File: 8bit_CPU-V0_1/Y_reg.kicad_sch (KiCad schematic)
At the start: 3 parts, among them U38 74LS04, U60 74LS574

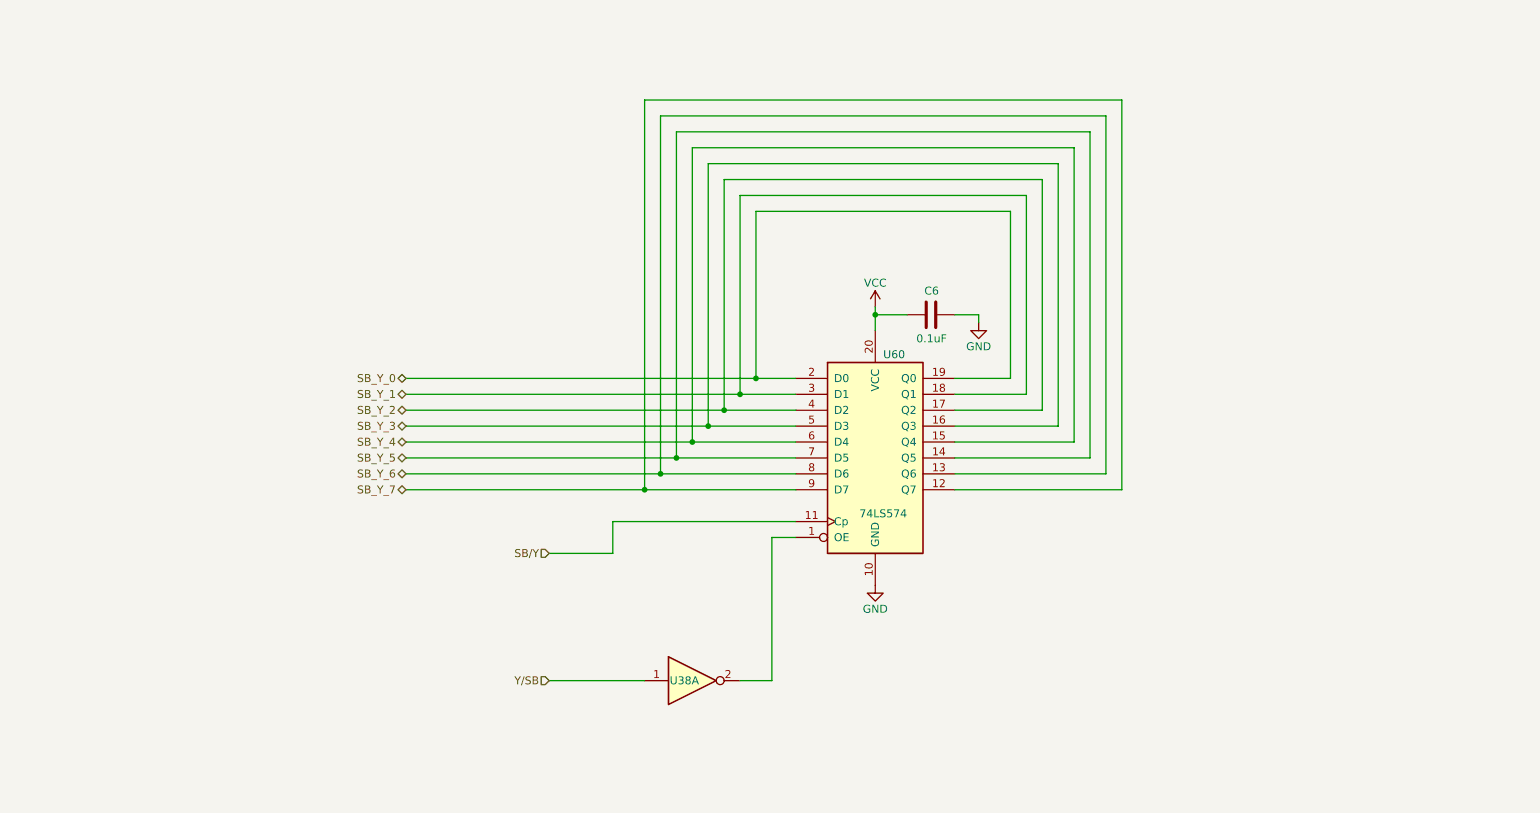
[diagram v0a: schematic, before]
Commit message: Update
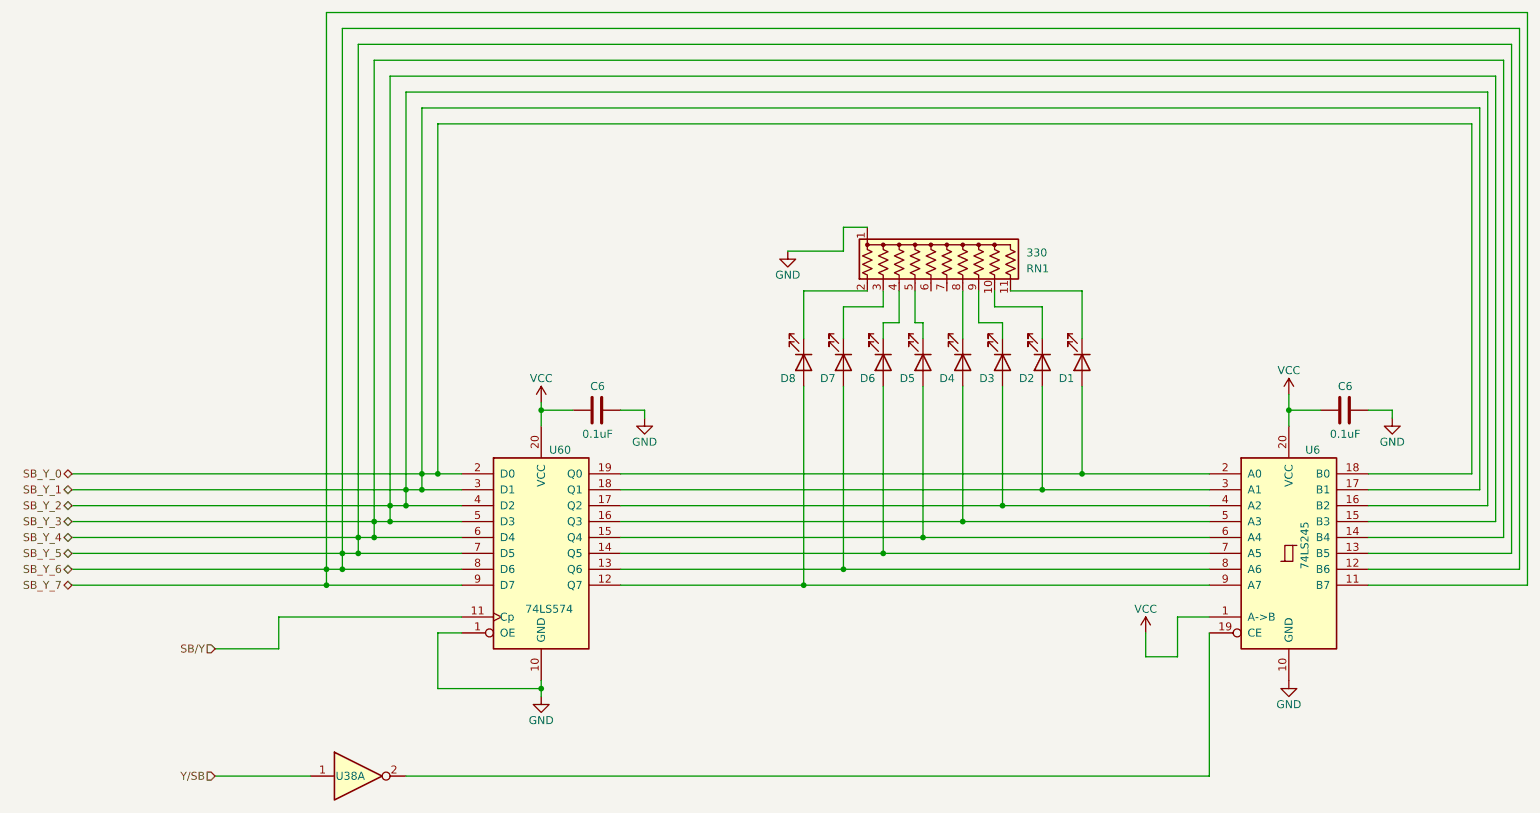
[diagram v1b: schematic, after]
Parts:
- added C6: 0.1uF, symbol Device:C
- added D1, D2, D3, D4, D5, D6, D7, D8: LED, symbol Device:LED
- added RN1: 330, Resistor_THT:R_Array_SIP11, symbol Device:R_Network10_US
- added U6: 74LS245, symbol 74xx:74LS245
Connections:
- net GND: now also U60.1 (OE), C6.2, RN1.1 (common), U6.10 (GND)
- net SB_Y_0: now also U60.3 (D1), U60.4 (D2), U60.5 (D3), U60.6 (D4), U60.7 (D5), U60.8 (D6), U60.9 (D7), U6.11 (B7), U6.12 (B6), U6.13 (B5), U6.14 (B4), U6.15 (B3), U6.16 (B2), U6.17 (B1), U6.18 (B0); no longer U60.19 (Q0)
- net VCC: now also C6.1, U6.1 (A->B), U6.20 (VCC)
- net at U38.2: now also U6.19 (CE); no longer U60.1 (OE)
- net SB_Y_1: no longer names the net of U60.18 (Q1)
- net SB_Y_1: now also D2.2 (A), U6.3 (A1); no longer U60.3 (D1)
- net SB_Y_2: no longer names the net of U60.17 (Q2)
- net SB_Y_2: now also D3.2 (A), U6.4 (A2); no longer U60.4 (D2)
- net SB_Y_3: no longer names the net of U60.16 (Q3)
- net SB_Y_3: now also D4.2 (A), U6.5 (A3); no longer U60.5 (D3)
- net SB_Y_4: no longer names the net of U60.15 (Q4)
- net SB_Y_4: now also D5.2 (A), U6.6 (A4); no longer U60.6 (D4)
- net SB_Y_5: no longer names the net of U60.14 (Q5)
- net SB_Y_5: now also D6.2 (A), U6.7 (A5); no longer U60.7 (D5)
- net SB_Y_6: no longer names the net of U60.13 (Q6)
- net SB_Y_6: now also D7.2 (A), U6.8 (A6); no longer U60.8 (D6)
- net SB_Y_7: no longer names the net of U60.12 (Q7)
- net SB_Y_7: now also D8.2 (A), U6.9 (A7); no longer U60.9 (D7)
- new net: D2.1 (K), RN1.10 (R9)
- new net: D1.1 (K), RN1.11 (R10)
- new net: D8.1 (K), RN1.2 (R1)
- new net: D7.1 (K), RN1.3 (R2)
- new net: D6.1 (K), RN1.4 (R3)
- new net: D5.1 (K), RN1.5 (R4)
- new net: D4.1 (K), RN1.8 (R7)
- new net: D3.1 (K), RN1.9 (R8)
- new net: D1.2 (A), U6.2 (A0), U60.19 (Q0)
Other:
- moved on the sheet: C6, U38A, U60
